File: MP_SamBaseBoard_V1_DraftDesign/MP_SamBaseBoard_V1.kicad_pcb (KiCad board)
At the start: 2 copper layers, 175 x 198.8 mm, 255 parts

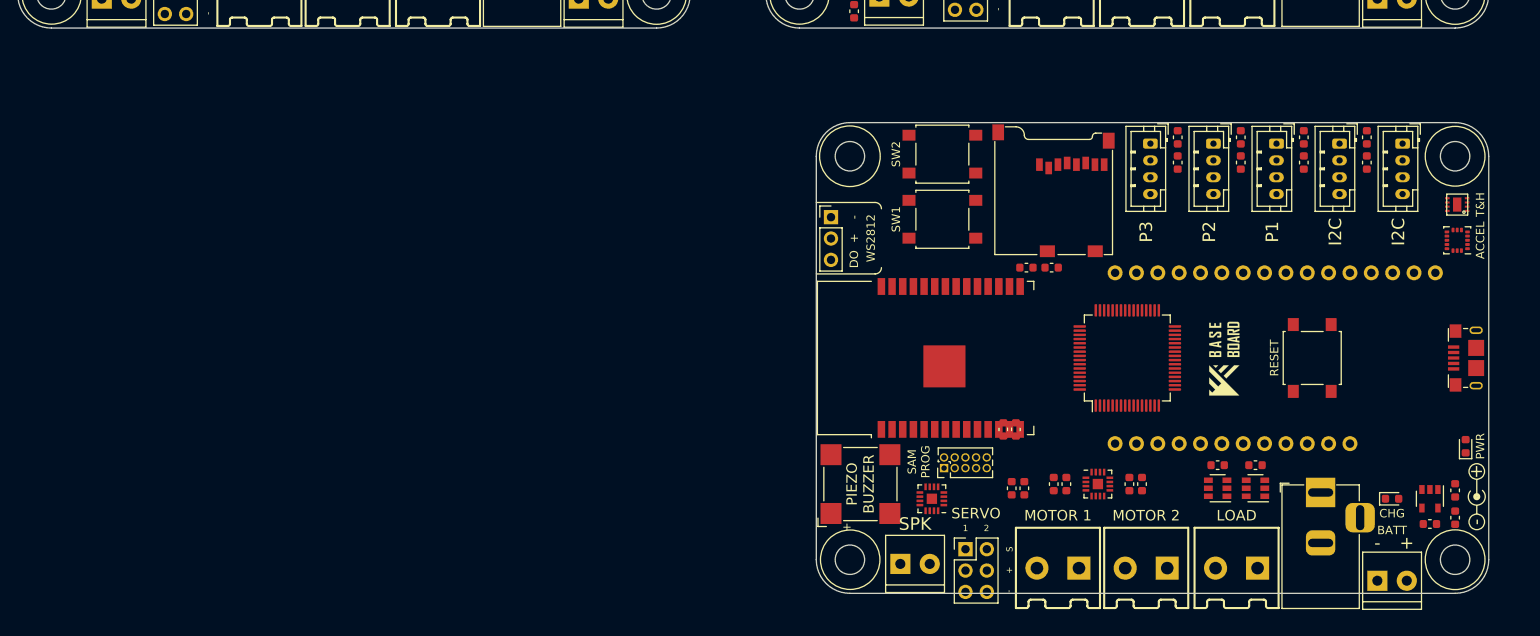
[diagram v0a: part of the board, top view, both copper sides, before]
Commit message: update
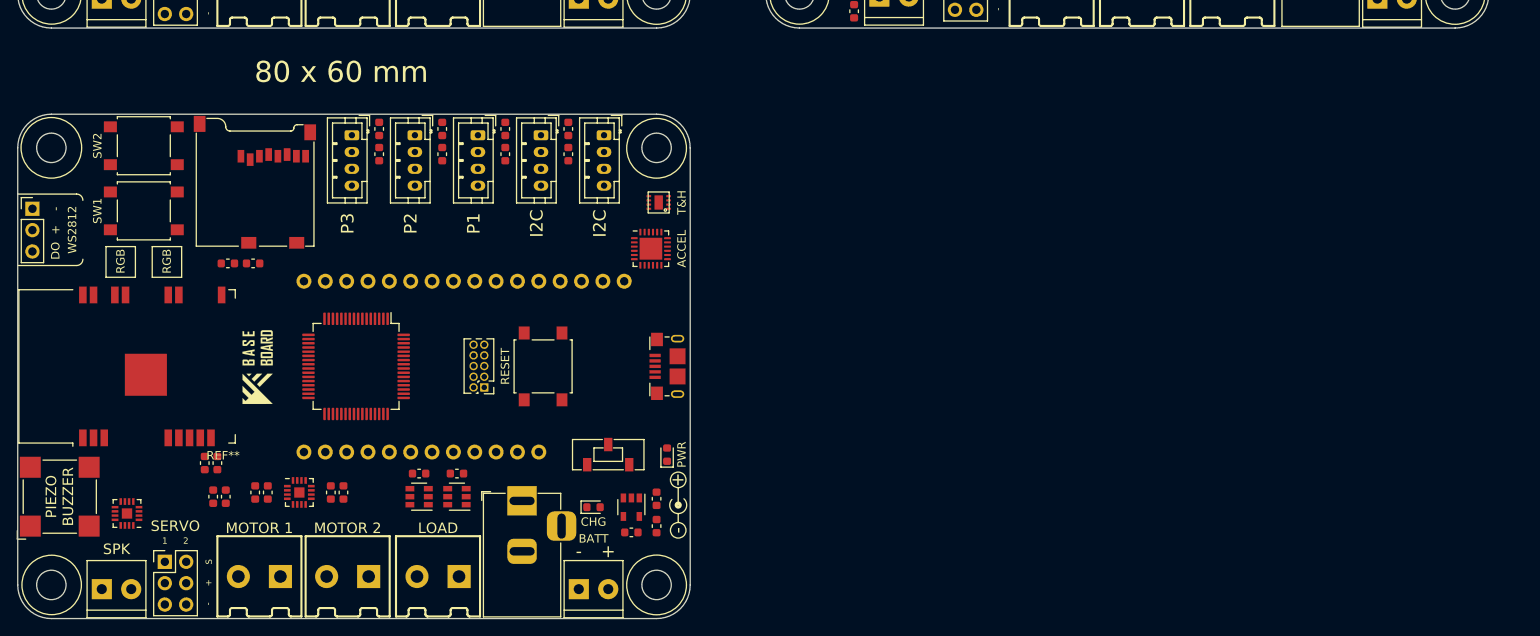
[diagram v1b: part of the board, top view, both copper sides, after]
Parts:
- removed the REF** at (333.2, 208.5)
- removed the REF** at (337.8, 211.5)
- removed the REF** at (340.8, 207.5)
- removed the REF** at (327.0, 166.2)
- removed the REF** at (289.5, 207.2)
- removed the REF** at (304.5, 166.2)
- removed the REF** at (322.8, 168.5)
- removed the REF** at (322.8, 165.5)
- removed the REF** at (312.0, 166.2)
- removed the REF** at (288.5, 200.2)
- removed the REF** at (342.0, 202.2)
- removed the REF** at (302.0, 206.8)
- removed the REF** at (307.8, 168.5)
- removed the REF** at (312.5, 207.2)
- removed the REF** at (280.8, 191.8)
- removed the REF** at (268.8, 167.8)
- removed the REF** at (304.0, 216.8)
- removed the REF** at (279.8, 175.2)
- removed the REF** at (279.8, 167.5)
- removed the REF** at (340.8, 210.8)
- removed the REF** at (294.5, 206.8)
- removed the REF** at (293.0, 206.8)
- removed the REF** at (315.2, 165.5)
- removed the REF** at (330.2, 165.5)
- removed the REF** at (298.2, 206.8)
- removed the REF** at (293.5, 216.8)
- removed the REF** at (288.0, 207.2)
- removed the REF** at (333.2, 218.2)
- removed the REF** at (303.5, 206.8)
- removed the REF** at (278.5, 208.5)
- removed the REF** at (268.8, 215.8)
- removed the REF** at (340.8, 215.8)
- removed the REF** at (317.0, 207.2)
- removed the REF** at (341.0, 177.8)
- removed the REF** at (334.5, 166.2)
- removed the REF** at (315.2, 168.5)
- removed the REF** at (287.0, 200.2)
- removed the REF** at (289.8, 181.0)
- removed the REF** at (312.5, 204.5)
- removed the REF** at (323.8, 191.8)
- removed the REF** at (330.2, 168.5)
- removed the REF** at (319.5, 166.2)
- removed the REF** at (317.0, 204.5)
- removed the REF** at (340.8, 167.8)
- removed the REF** at (314.8, 216.8)
- removed the REF** at (292.8, 181.0)
- removed the REF** at (307.8, 165.5)
- removed the REF** at (276.5, 216.2)
- added REF**: SW_SPDT_CK-JS102011JCQN, GiraffeTech-Electromechanical:SW_SPDT_CK-JS102011JCQN, F.Cu at (240.0, 203.2)
- added REF**: C_0603_1608Metric, Capacitor_SMD:C_0603_1608Metric, F.Cu at (208.5, 207.8)
- added REF**: C_0603_1608Metric, Capacitor_SMD:C_0603_1608Metric, F.Cu at (220.2, 164.5)
- added REF**: SOT-23-6, Package_TO_SOT_SMD:SOT-23-6, F.Cu at (222.0, 208.2)
- added REF**: C_0603_1608Metric, Capacitor_SMD:C_0603_1608Metric, F.Cu at (242.8, 212.5)
- added REF**: R_0603_1608Metric, Resistor_SMD:R_0603_1608Metric, F.Cu at (192.0, 204.2)
- added REF**: QFN-16-1EP_3x3mm_Pitch0.5mm, GiraffeTech-Maxim:QFN-16-1EP_3x3mm_Pitch0.5mm, F.Cu at (203.2, 207.8)
- added REF**: R_0603_1608Metric, Resistor_SMD:R_0603_1608Metric, F.Cu at (217.5, 205.5)
- added REF**: DINKLE_EK500V-2P, GiraffeTech-Connector:DINKLE_EK500V-2P, F.Cu at (209.0, 217.8)
- added REF**: R_0603_1608Metric, Resistor_SMD:R_0603_1608Metric, F.Cu at (222.0, 205.5)
- added REF**: SOT-23-6, Package_TO_SOT_SMD:SOT-23-6, F.Cu at (217.5, 208.2)
- added REF**: MountingHole_3.5mm, MountingHole:MountingHole_3.5mm, F.Cu at (173.8, 166.8)
- added REF**: C_0603_1608Metric, Capacitor_SMD:C_0603_1608Metric, F.Cu at (199.5, 207.8)
- added REF**: JST_PH_B4B-PH-K_1x04_P2.00mm_Vertical, Connector_JST:JST_PH_B4B-PH-K_1x04_P2.00mm_Vertical, F.Cu at (217.0, 165.2)
- added REF**: LED_0603_1608Metric, LED_SMD:LED_0603_1608Metric, F.Cu at (247.0, 203.2)
- added REF**: C_0603_1608Metric, Capacitor_SMD:C_0603_1608Metric, F.Cu at (235.2, 167.5)
- added REF**: C_0603_1608Metric, Capacitor_SMD:C_0603_1608Metric, F.Cu at (235.2, 164.5)
- added REF**: C_0603_1608Metric, Capacitor_SMD:C_0603_1608Metric, F.Cu at (220.2, 167.5)
- added REF**: MountingHole_3.5mm, MountingHole:MountingHole_3.5mm, F.Cu at (245.8, 166.8)
- added REF**: C_0603_1608Metric, Capacitor_SMD:C_0603_1608Metric, F.Cu at (194.5, 208.2)
- added REF**: JST_PH_B4B-PH-K_1x04_P2.00mm_Vertical, Connector_JST:JST_PH_B4B-PH-K_1x04_P2.00mm_Vertical, F.Cu at (209.5, 165.2)
- added REF**: MountingHole_3.5mm, MountingHole:MountingHole_3.5mm, F.Cu at (245.8, 218.8)
- added REF**: C_0603_1608Metric, Capacitor_SMD:C_0603_1608Metric, F.Cu at (193.0, 208.2)
- added REF**: SW_SPST_B3S-1000, Button_Switch_SMD:SW_SPST_B3S-1000, F.Cu at (184.8, 174.2)
- added REF**: LED_0603_1608Metric, LED_SMD:LED_0603_1608Metric, F.Cu at (238.2, 209.5)
- added REF**: C_0603_1608Metric, Capacitor_SMD:C_0603_1608Metric, F.Cu at (198.0, 207.8)
- added REF**: C_0603_1608Metric, Capacitor_SMD:C_0603_1608Metric, F.Cu at (212.8, 164.5)
- added REF**: C_0603_1608Metric, Capacitor_SMD:C_0603_1608Metric, F.Cu at (212.8, 167.5)
- added REF**: Dinkle_ED350V_2Pins_Pitch3.5mm, GiraffeTech-Connector:TerminalBlock_Dinkle_ED350V_1x02_P3.50mm_Horizontal, F.Cu at (181.5, 219.2)
- added REF**: C_0603_1608Metric, Capacitor_SMD:C_0603_1608Metric, F.Cu at (227.8, 164.5)
- added REF**: JST_PH_B4B-PH-K_1x04_P2.00mm_Vertical, Connector_JST:JST_PH_B4B-PH-K_1x04_P2.00mm_Vertical, F.Cu at (239.5, 165.2)
- added REF**: C_0603_1608Metric, Capacitor_SMD:C_0603_1608Metric, F.Cu at (245.8, 208.5)
- added REF**: SW_SPST_B3S-1000, Button_Switch_SMD:SW_SPST_B3S-1000, F.Cu at (232.2, 192.8)
- added REF**: DINKLE_EK500V-2P, GiraffeTech-Connector:DINKLE_EK500V-2P, F.Cu at (198.5, 217.8)
- added REF**: C_0603_1608Metric, Capacitor_SMD:C_0603_1608Metric, F.Cu at (194.8, 180.5)
- added REF**: DINKLE_EK500V-2P, GiraffeTech-Connector:DINKLE_EK500V-2P, F.Cu at (219.8, 217.8)
- added REF**: R_0603_1608Metric, Resistor_SMD:R_0603_1608Metric, F.Cu at (193.5, 204.2)
- added REF**: C_0603_1608Metric, Capacitor_SMD:C_0603_1608Metric, F.Cu at (207.0, 207.8)
- added REF**: C_0603_1608Metric, Capacitor_SMD:C_0603_1608Metric, F.Cu at (197.8, 180.5)
- added REF**: JST_PH_B4B-PH-K_1x04_P2.00mm_Vertical, Connector_JST:JST_PH_B4B-PH-K_1x04_P2.00mm_Vertical, F.Cu at (224.5, 165.2)
- added REF**: QFN-24-1EP_4x4mm_P0.5mm_EP2.7x2.6mm, Package_DFN_QFN:QFN-24-1EP_4x4mm_P0.5mm_EP2.7x2.6mm, F.Cu at (245.1, 178.8)
- added REF**: ESP32-WROOM-32_WifiNinaPin, GiraffeTech-NodeMCU:ESP32-WROOM-32_WifiNinaPin, F.Cu at (185.8, 192.8)
- added REF**: MountingHole_3.5mm, MountingHole:MountingHole_3.5mm, F.Cu at (173.8, 218.8)
- added REF**: Dinkle_ED350V_2Pins_Pitch3.5mm, GiraffeTech-Connector:TerminalBlock_Dinkle_ED350V_1x02_P3.50mm_Horizontal, F.Cu at (238.2, 219.2)
- added REF**: C_0603_1608Metric, Capacitor_SMD:C_0603_1608Metric, F.Cu at (227.8, 167.5)
- added REF**: SW_SPST_B3S-1000, Button_Switch_SMD:SW_SPST_B3S-1000, F.Cu at (184.8, 166.5)
- added REF**: JST_PH_B4B-PH-K_1x04_P2.00mm_Vertical, Connector_JST:JST_PH_B4B-PH-K_1x04_P2.00mm_Vertical, F.Cu at (232.0, 165.2)
- added REF**: QFN-16-1EP_3x3mm_Pitch0.5mm, GiraffeTech-Maxim:QFN-16-1EP_3x3mm_Pitch0.5mm, F.Cu at (182.8, 210.2)
- added REF**: C_0603_1608Metric, Capacitor_SMD:C_0603_1608Metric, F.Cu at (245.8, 211.8)
- moved G*** 115.0 mm to (198.2, 192.8)
- moved MS2 96.5 mm to (248.2, 181.3)
- moved REF** 95.3 mm to (174.8, 208.2)
- moved REF** 95.3 mm to (187.2, 216.0)
- moved REF** 95.0 mm to (171.5, 174.0)
- moved REF** 95.0 mm to (204.0, 167.8)
- moved REF** 95.0 mm to (248.2, 209.2)
- moved REF** 95.0 mm to (248.2, 192.8)
- moved REF** 95.0 mm to (242.8, 209.5)
- moved REF** 95.0 mm to (229.8, 208.8)
- moved REF** 95.0 mm to (246.0, 173.2)
- moved REF** 91.8 mm to (210.0, 192.8), turned to 270 degrees
- moved REF** 55.5 mm to (225.2, 195.2), turned to 180 degrees
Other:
- board size 175 x 198.8 mm -> 175 x 201.8 mm
